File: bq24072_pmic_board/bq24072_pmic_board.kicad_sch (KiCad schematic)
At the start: 14 parts, among them J101 USB_B_Micro, J102 Battery, J103 Conn_01x04_Female, U101 AMS1117-3.3

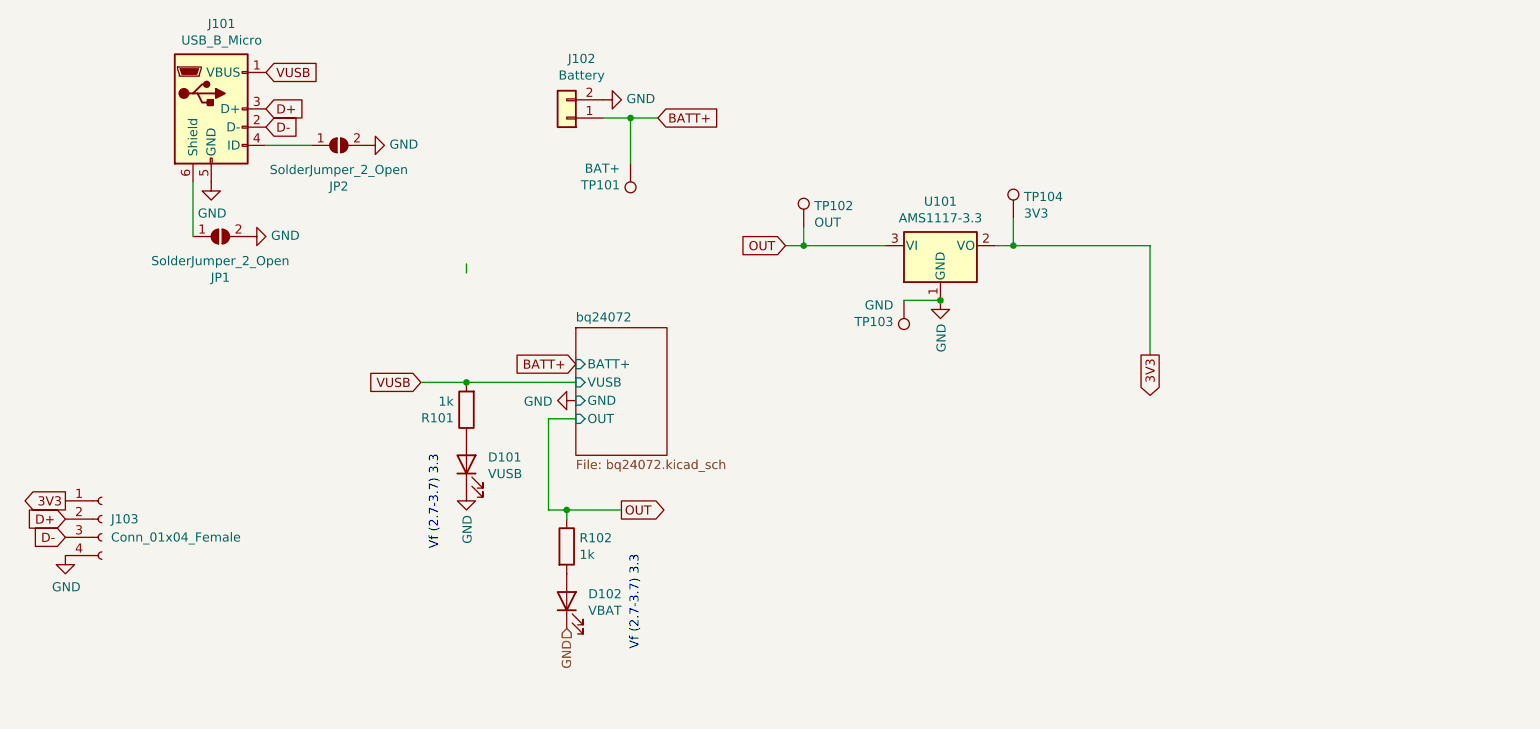
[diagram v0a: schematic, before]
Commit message: final touches + v1 jlcpcb fab files
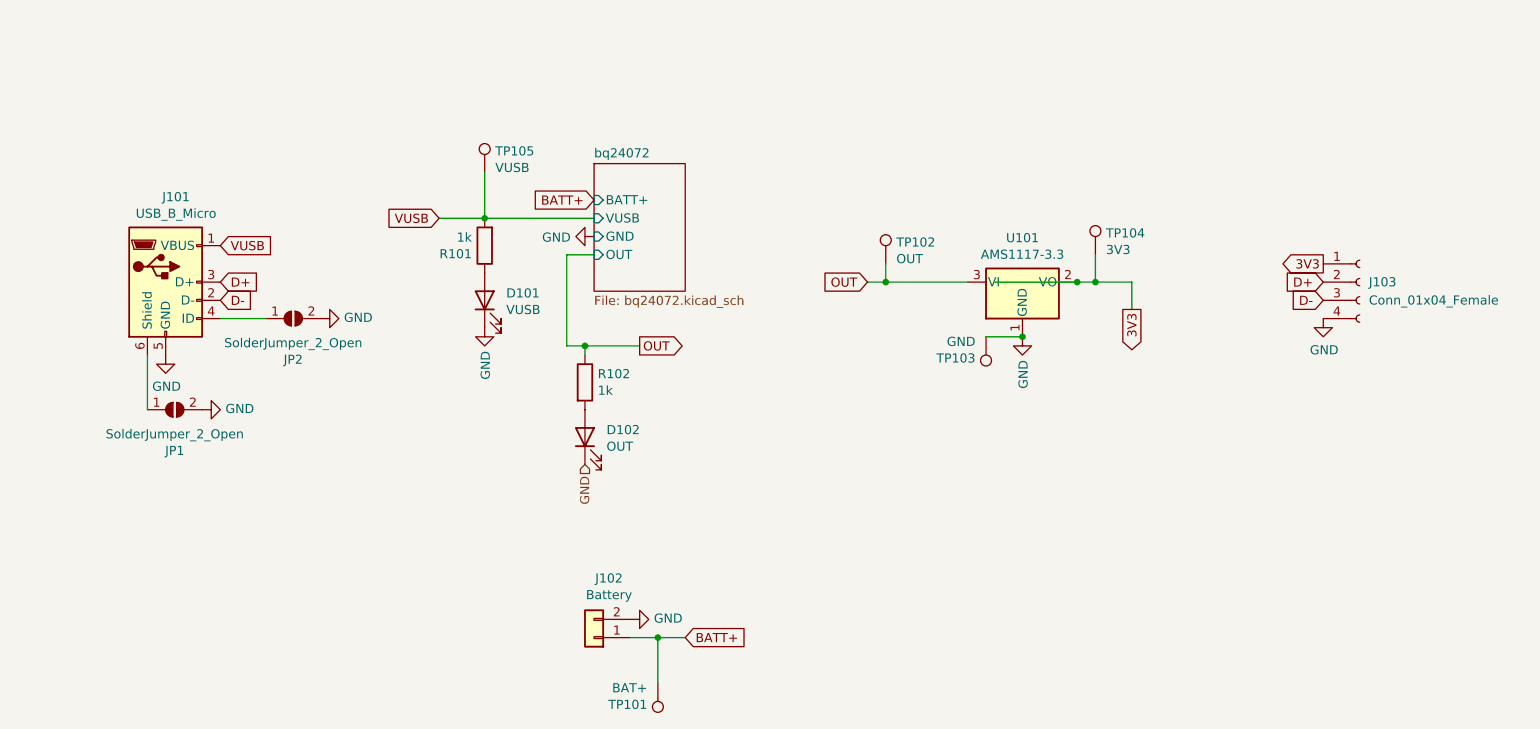
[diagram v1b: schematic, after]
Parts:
- added TP105: VUSB, TestPoint:TestPoint_Pad_D2.0mm, symbol Connector:TestPoint
- D102: value VBAT -> OUT
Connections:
- net VUSB: now also TP105.1
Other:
- note removed: "Vf (2.7-3.7) 3.3"
- moved on the sheet: D101, D102, J101, J102, J103, JP1, JP2, R101, R102, TP101, TP102, TP103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
